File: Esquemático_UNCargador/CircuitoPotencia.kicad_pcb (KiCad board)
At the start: 2 copper layers, 28.4 x 71.9 mm, 56 parts, among them IC1 LF353, J1 Conn_01x08_Pin, J2 Relay1, J3 Conn_02x03_Counter_Clockwise, J4 GFCI, J5 PZEM 004T 100A, J6 NTC 3950, J8 Conn_01x02_Pin, J9 Relay2, Q1 PN2222A, Q2 PN2222A, SW1 SW_Push, SW2 SW_Push, SW3 SW_Push, SW4 SW_Push, SW5 SW_Push, U3 LM7912(Inversor)

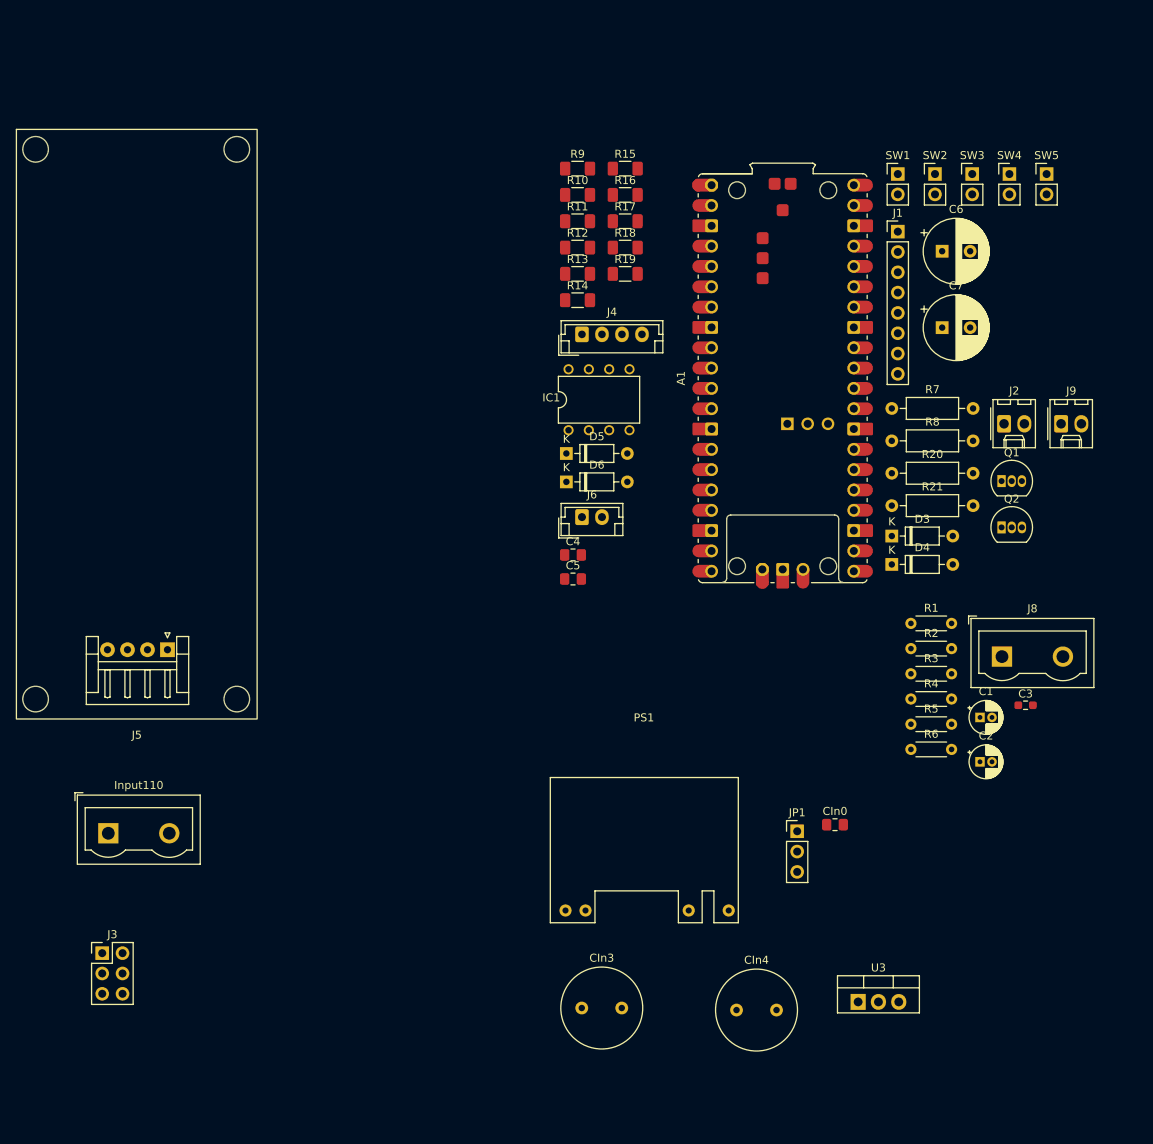
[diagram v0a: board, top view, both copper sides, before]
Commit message: version inicial layout PCB
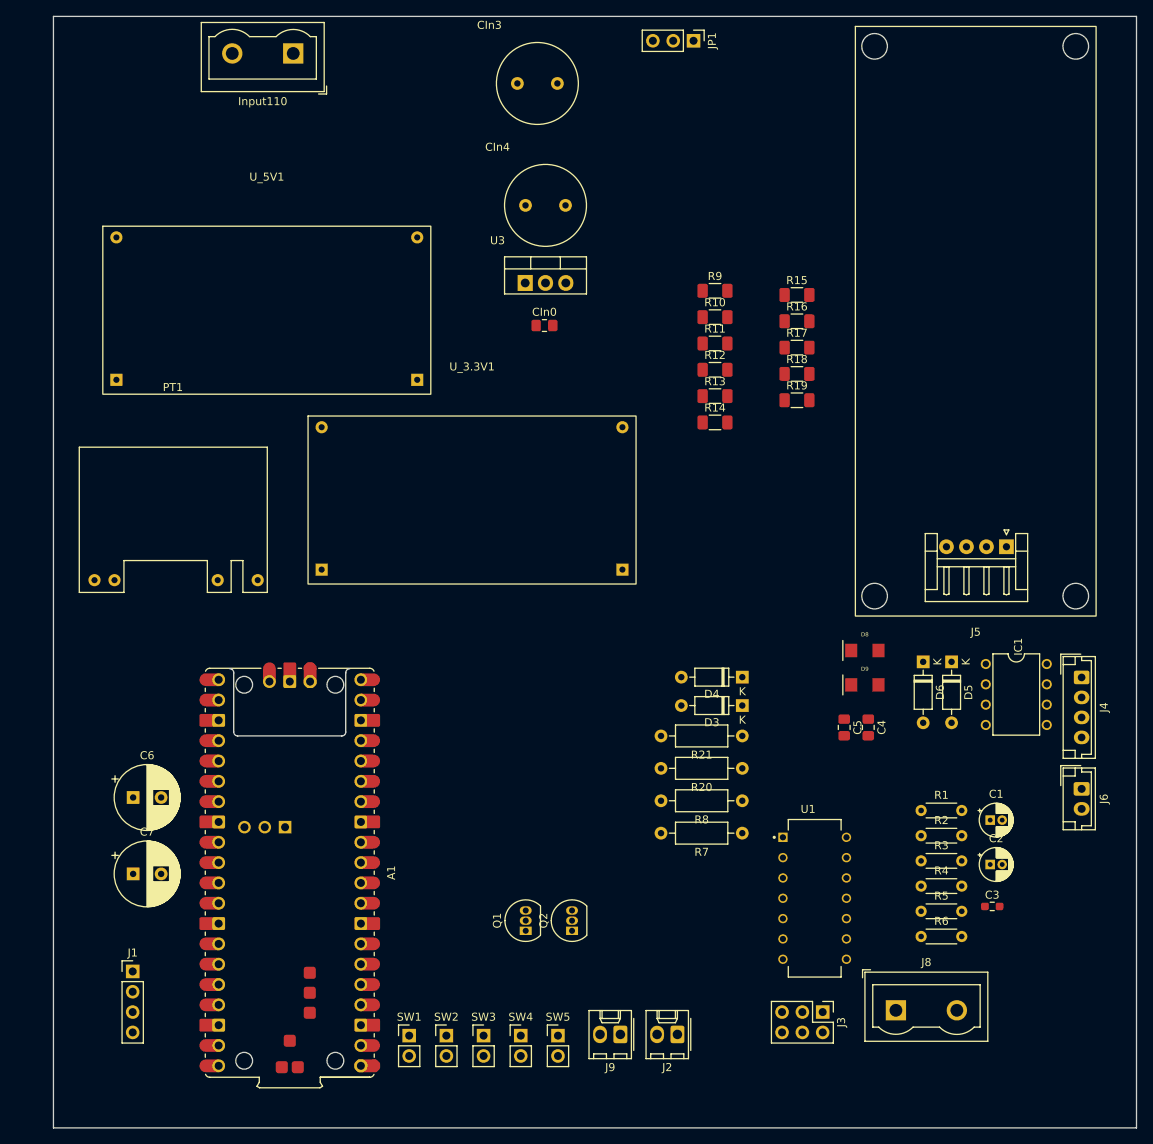
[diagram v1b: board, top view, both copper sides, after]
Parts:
- removed PS1: BAC05S05DC, Convertidor_AC-DC:AC-DC_Converter
- added D8: SMAZ5V1, Esquemático_UNCargador:DO-214AC, F.Cu at (146.9, 94.8)
- added D9: SMAZ5V1, Esquemático_UNCargador:DO-214AC, F.Cu at (146.9, 99.1)
- added PT1: BAC05S05DC, Convertidor_AC-DC:AC-DC_Converter, F.Cu at (60.2, 77.0)
- added U1: LM324N, LM324:DIP794W45P254L1969H508Q14, F.Cu at (140.6, 125.7)
- added U_3.3V1: LM2596_3.3V, LM2596ADJ:LM2596ADJ, F.Cu at (97.8, 69.4)
- added U_5V1: LM2596_5V, LM2596ADJ:LM2596ADJ, F.Cu at (72.1, 45.7)
- J1: value Conn_01x08_Pin -> Conn_01x04_Pin; footprint Connector_PinHeader_2.54mm:PinHeader_1x08_P2.54mm_Vertical -> Connector_PinHeader_2.54mm:PinHeader_1x04_P2.54mm_Vertical
- moved J1 133.0 mm to (55.4, 134.9)
- moved SW1 123.8 mm to (89.9, 142.9)
- moved SW2 123.8 mm to (94.6, 142.9)
- moved SW3 123.8 mm to (99.2, 142.9)
- moved SW4 123.8 mm to (103.9, 142.9)
- moved SW5 123.8 mm to (108.5, 142.9)
- moved C6 122.0 mm to (55.4, 113.1)
- moved C7 122.0 mm to (55.4, 122.7)
- moved A1 118.5 mm to (83.9, 146.7), turned to 180 degrees
- moved CIn3 115.8 mm to (103.5, 23.9)
- moved J5 105.7 mm to (160.8, 92.9)
- moved CIn4 104.0 mm to (104.5, 39.1)
- moved Input110 100.2 mm to (75.4, 20.1), turned to 180 degrees
- moved JP1 99.7 mm to (125.5, 18.5), turned to -90 degrees
- moved U3 99.0 mm to (104.4, 48.8)
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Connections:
- net CLK renamed DIsplaySCL
- J1 pad 3: SDA -> DisplaySDA
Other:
- board size 28.4 x 71.9 mm -> 135.4 x 138.9 mm
